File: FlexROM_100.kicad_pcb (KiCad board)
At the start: 2 copper layers, 16.4 x 34.2 mm, 6 parts, among them J1 LH535618 DIP LEGS, J2 ~WE~, U1 28C256

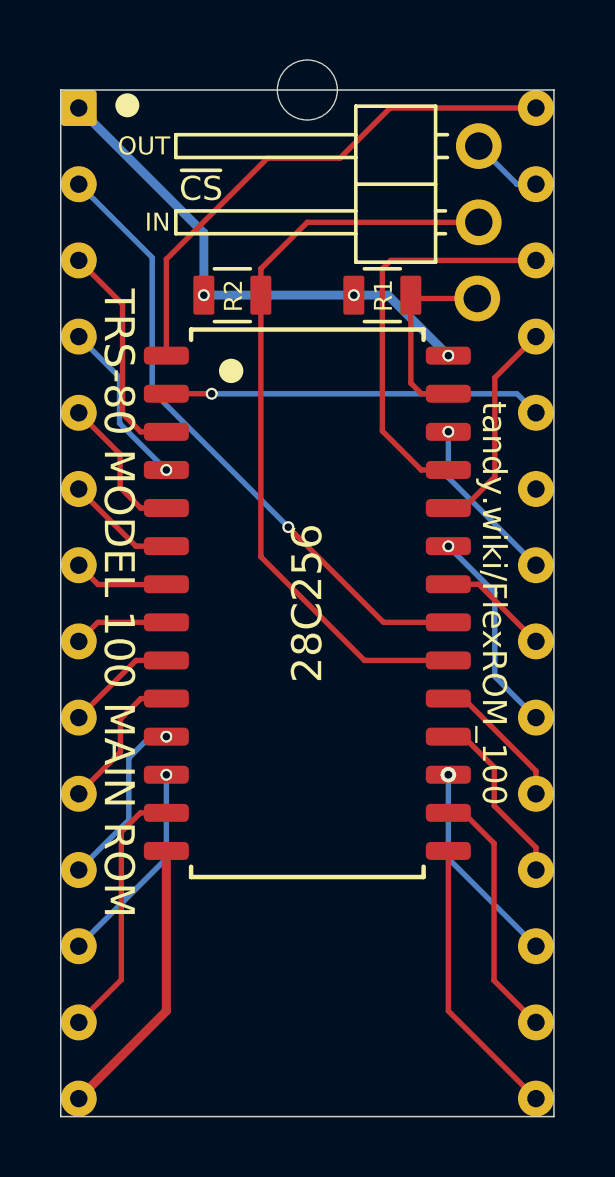
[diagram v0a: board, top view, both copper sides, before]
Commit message: silkscreen
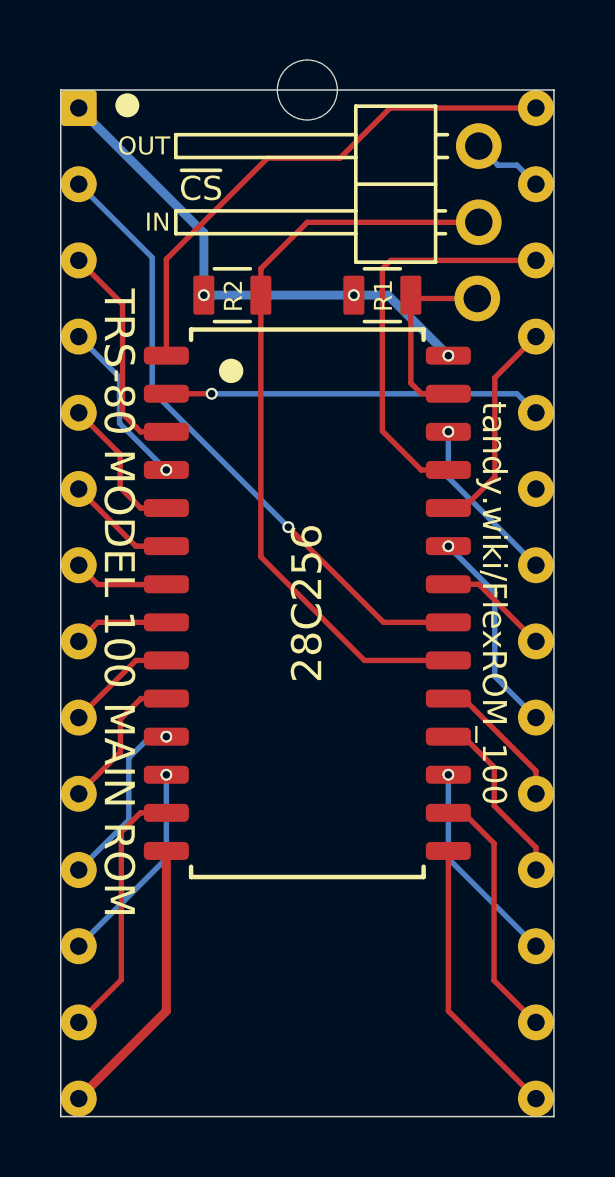
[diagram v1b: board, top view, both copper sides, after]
